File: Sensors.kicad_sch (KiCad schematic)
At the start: 22 parts, among them IC1 ICM-42688-P, IC2 W25Q256JWPIQ, U2 DPS310, U3 AT7456E

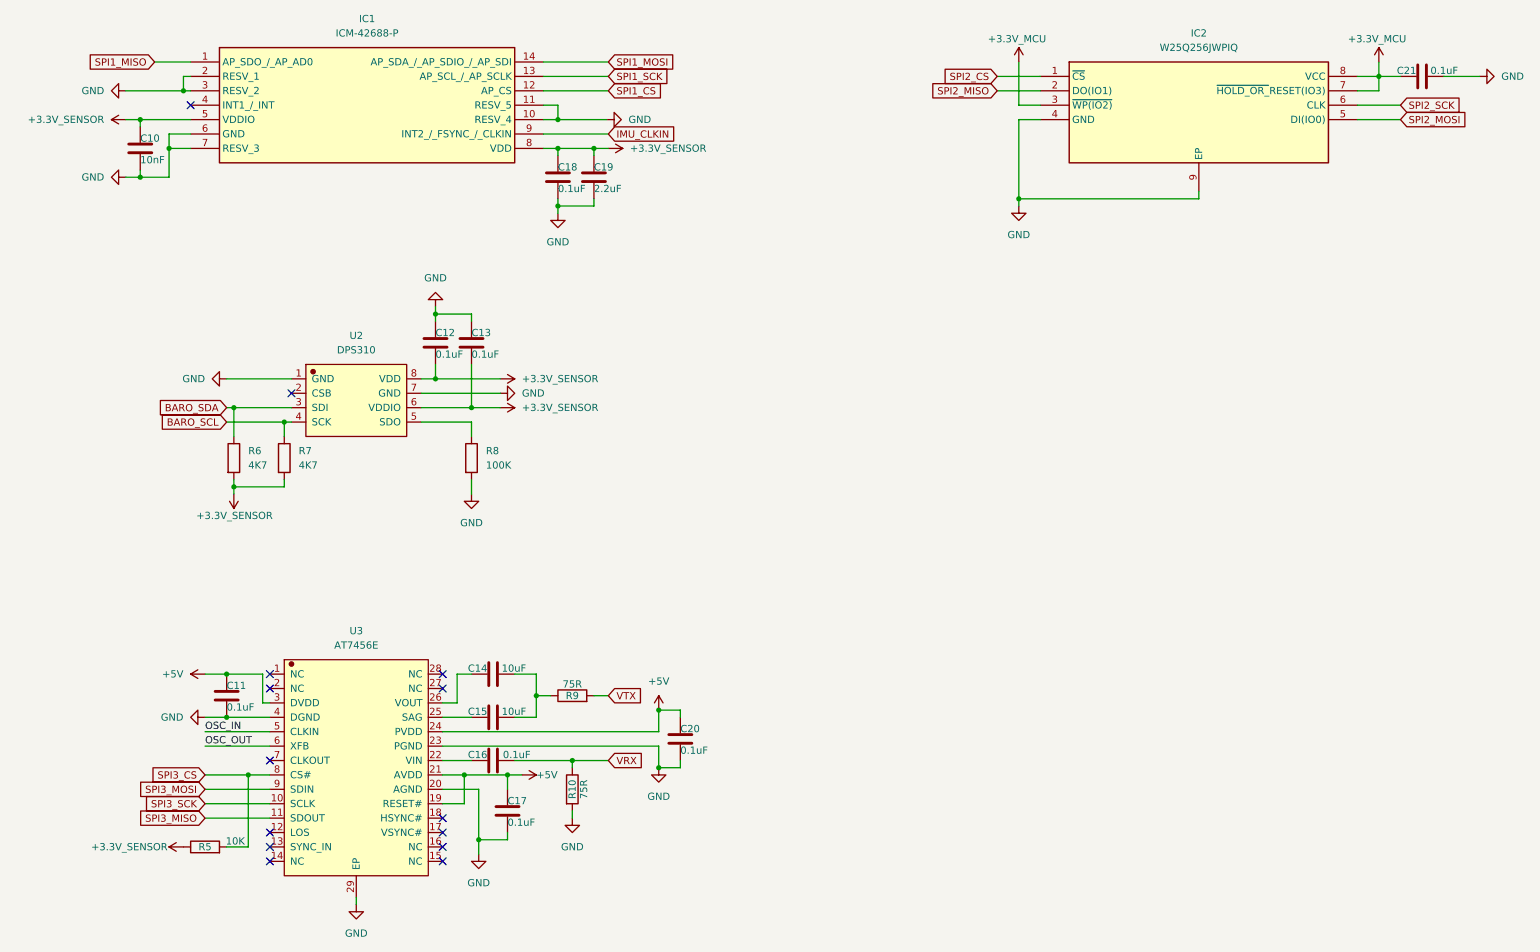
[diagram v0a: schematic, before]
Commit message: Finished SCH
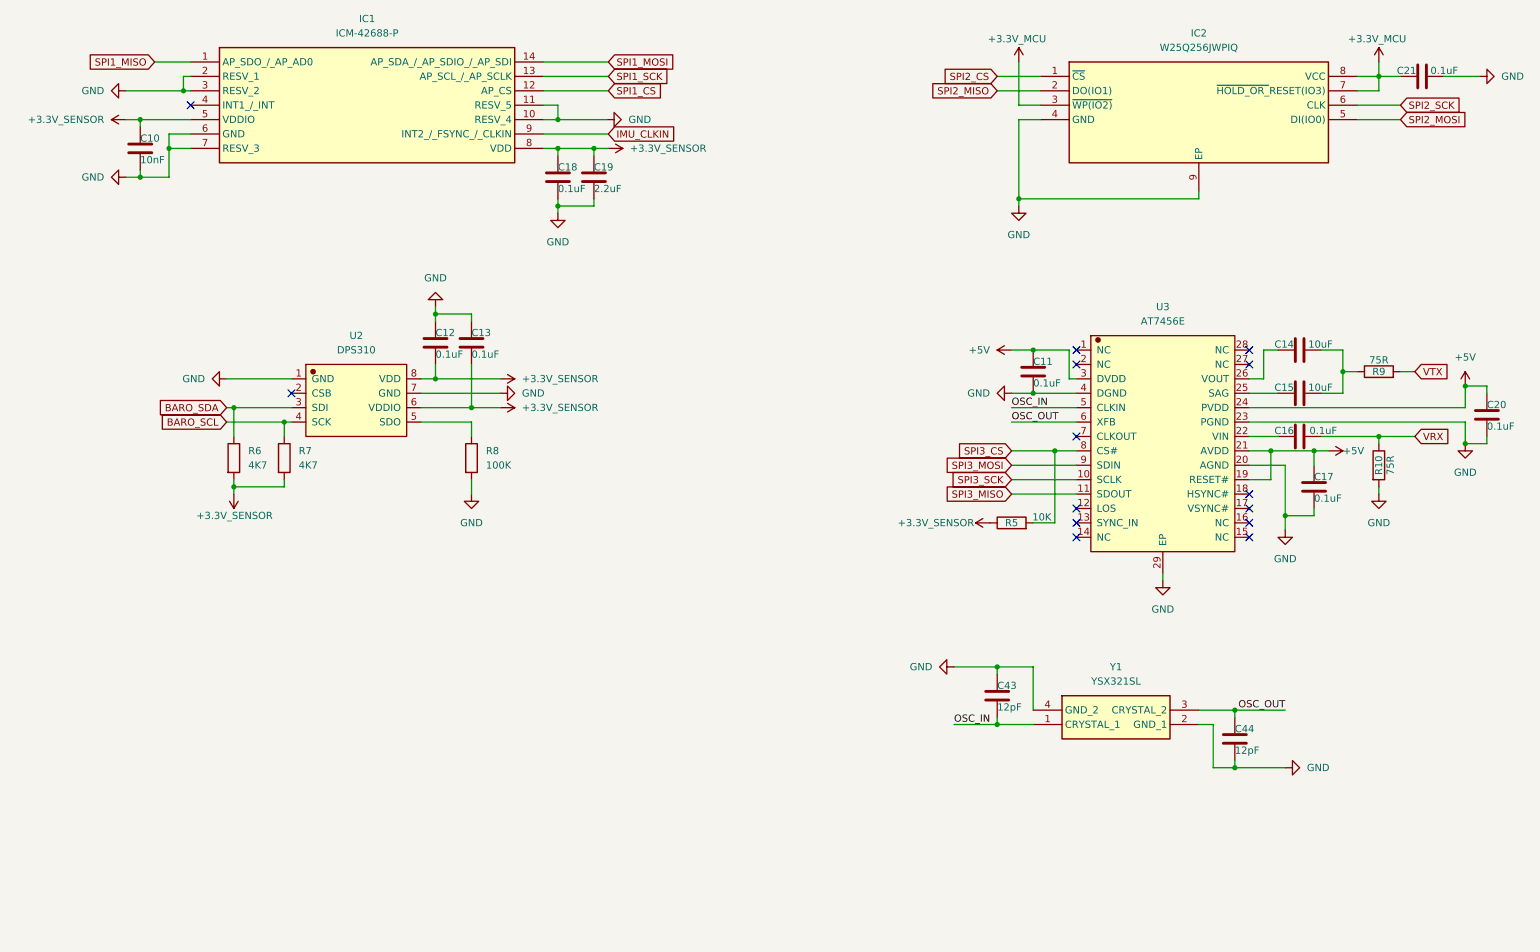
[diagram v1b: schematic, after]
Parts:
- added C43, C44: 12pF, Capacitor_SMD:C_0402_1005Metric, symbol Library:C
- added Y1: YSX321SL, YSX321SL, symbol SamacSys_Parts:YSX321SL
- C10, C11, C12, C13, C14, C15, C16, C17, C18, C19, C20, C21: footprint (none) -> Capacitor_SMD:C_0402_1005Metric
- R10, R5, R6, R7, R8, R9: footprint (none) -> Resistor_SMD:R_0402_1005Metric
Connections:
- net GND: now also C43.1, C44.2, Y1.2 (GND_1), Y1.4 (GND_2)
- net OSC_IN: now also C43.2, Y1.1 (CRYSTAL_1)
- net OSC_OUT: now also C44.1, Y1.3 (CRYSTAL_2)
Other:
- moved on the sheet: C11, C14, C15, C16, C17, C20, R10, R5, R9, U3
